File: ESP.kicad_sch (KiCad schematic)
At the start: 13 parts, among them J1 Conn_01x03, SW1 SW_Push, U1 RP2040, U5 W25X40CLSS, U6 DRV8833PW, U7 DRV8833PW, U8 DRV8833PW

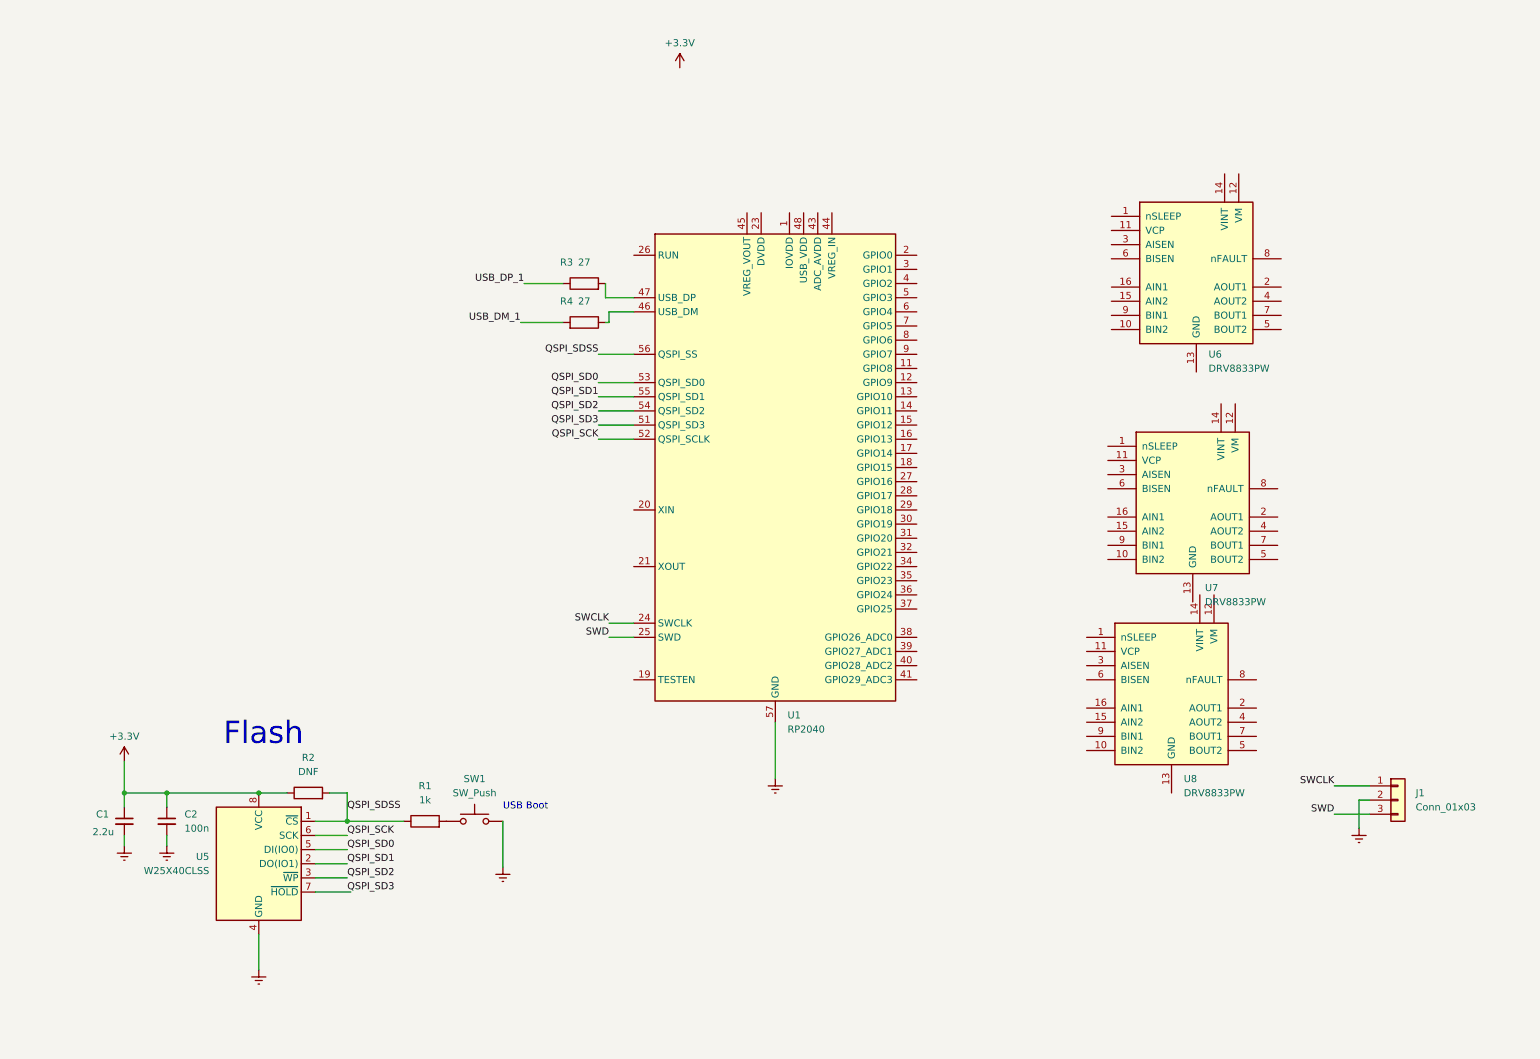
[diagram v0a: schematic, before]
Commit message: More progress
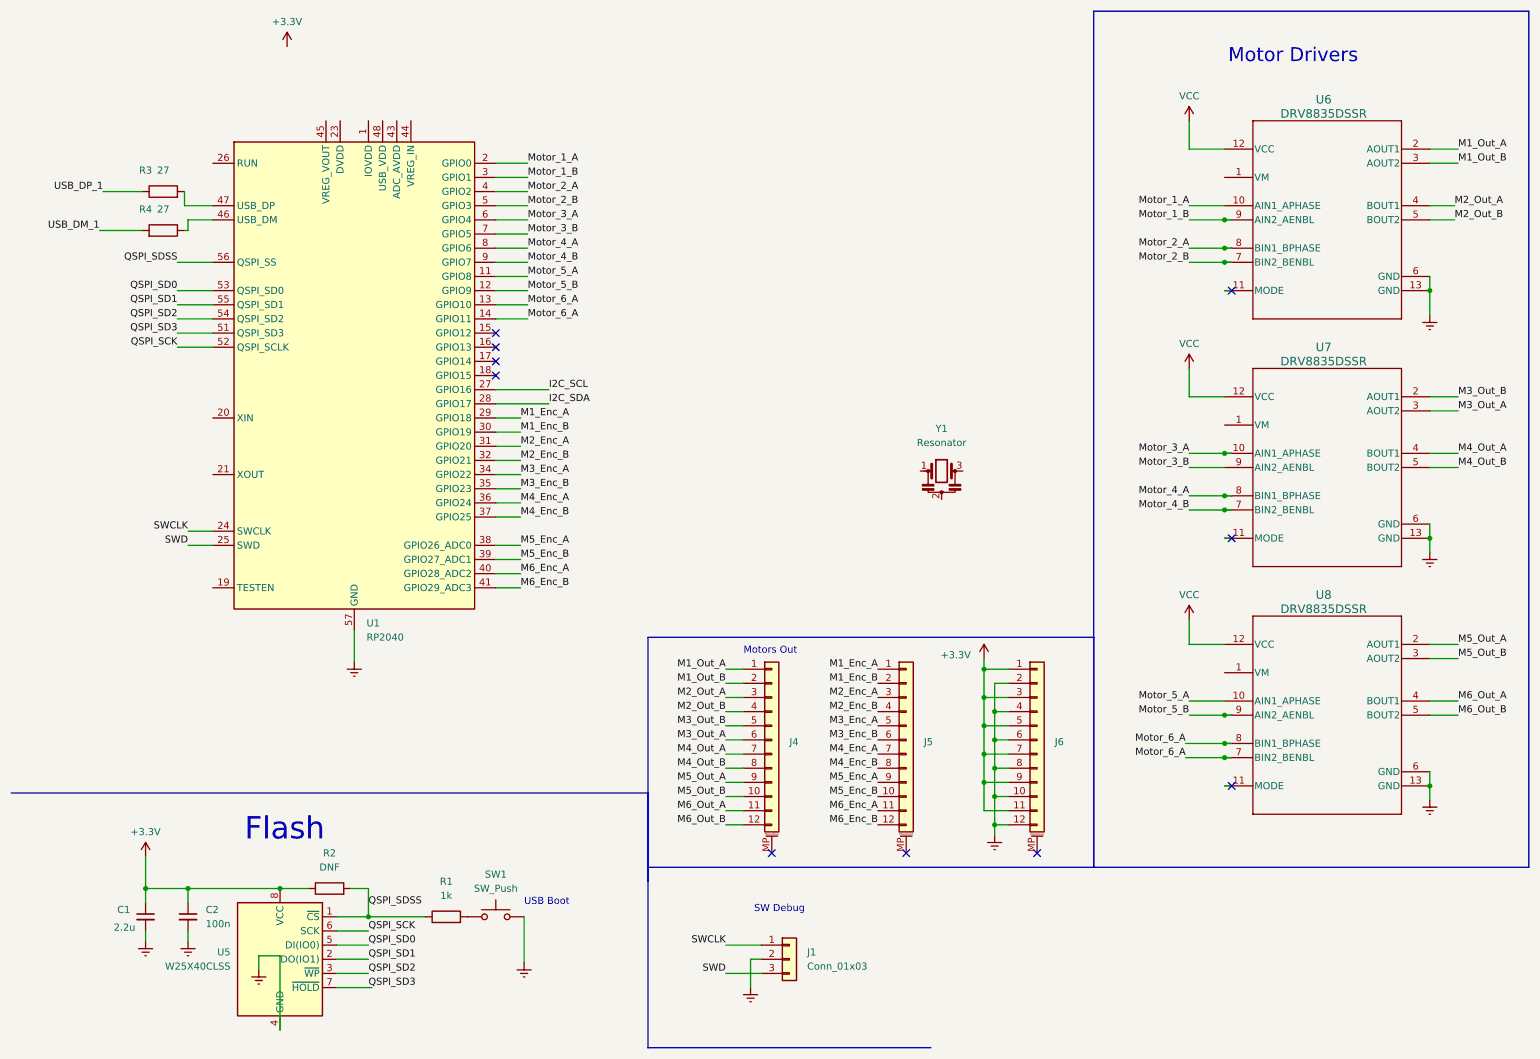
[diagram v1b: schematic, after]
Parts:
- removed U6, U7, U8: DRV8833PW, Package_SO:TSSOP-16_4.4x5mm_P0.65mm, symbol Driver_Motor:DRV8833PW
- added J4, J5, J6: Conn_01x12_MountingPin, symbol Connector_Generic_MountingPin:Conn_01x12_MountingPin
- added U6, U7, U8: DRV8835DSSR, DSS0012A, symbol DRV8835:DRV8835DSSR
- added Y1: Resonator, symbol Device:Resonator
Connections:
- net +3.3V: now also J6.1 (Pin_1), J6.11 (Pin_11), J6.3 (Pin_3), J6.5 (Pin_5), J6.7 (Pin_7), J6.9 (Pin_9)
- net Earth: now also J6.10 (Pin_10), J6.12 (Pin_12), J6.2 (Pin_2), J6.4 (Pin_4), J6.6 (Pin_6), J6.8 (Pin_8), U6.13 (GND), U6.6 (GND), U7.13 (GND), U7.6 (GND), U8.13 (GND), U8.6 (GND)
- net Motor_5_A: now reaches U1.11 (GPIO8)
- net Motor_5_A: now also U8.10 (AIN1_APHASE)
- net Motor_5_B: now reaches U1.12 (GPIO9)
- net Motor_5_B: now also U8.9 (AIN2_AENBL)
- net Motor_6_A: now reaches U1.13 (GPIO10)
- net Motor_6_A: now also U1.14 (GPIO11), U8.7 (BIN2_BENBL), U8.8 (BIN1_BPHASE)
- net Motor_1_A: now reaches U1.2 (GPIO0)
- net Motor_1_A: now also U6.10 (AIN1_APHASE)
- net I2C_SCL: now reaches U1.27 (GPIO16)
- net I2C_SDA: now reaches U1.28 (GPIO17)
- net M1_Enc_A: now reaches U1.29 (GPIO18)
- net M1_Enc_A: now also J5.1 (Pin_1)
- net Motor_1_B: now reaches U1.3 (GPIO1)
- net Motor_1_B: now also U6.9 (AIN2_AENBL)
- net M1_Enc_B: now reaches U1.30 (GPIO19)
- net M1_Enc_B: now also J5.2 (Pin_2)
- net M2_Enc_A: now reaches U1.31 (GPIO20)
- net M2_Enc_A: now also J5.3 (Pin_3)
- net M2_Enc_B: now reaches U1.32 (GPIO21)
- net M2_Enc_B: now also J5.4 (Pin_4)
- net M3_Enc_A: now reaches U1.34 (GPIO22)
- net M3_Enc_A: now also J5.5 (Pin_5)
- net M3_Enc_B: now reaches U1.35 (GPIO23)
- net M3_Enc_B: now also J5.6 (Pin_6)
- net M4_Enc_A: now reaches U1.36 (GPIO24)
- net M4_Enc_A: now also J5.7 (Pin_7)
- net M4_Enc_B: now reaches U1.37 (GPIO25)
- net M4_Enc_B: now also J5.8 (Pin_8)
- net M5_Enc_A: now reaches U1.38 (GPIO26_ADC0)
- net M5_Enc_A: now also J5.9 (Pin_9)
- net M5_Enc_B: now reaches U1.39 (GPIO27_ADC1)
- net M5_Enc_B: now also J5.10 (Pin_10)
- net Motor_2_A: now reaches U1.4 (GPIO2)
- net Motor_2_A: now also U6.8 (BIN1_BPHASE)
- net M6_Enc_A: now reaches U1.40 (GPIO28_ADC2)
- net M6_Enc_A: now also J5.11 (Pin_11)
- net M6_Enc_B: now reaches U1.41 (GPIO29_ADC3)
- net M6_Enc_B: now also J5.12 (Pin_12)
- net Motor_2_B: now reaches U1.5 (GPIO3)
- net Motor_2_B: now also U6.7 (BIN2_BENBL)
- net Motor_3_A: now reaches U1.6 (GPIO4)
- net Motor_3_A: now also U7.10 (AIN1_APHASE)
- net Motor_3_B: now reaches U1.7 (GPIO5)
- net Motor_3_B: now also U7.9 (AIN2_AENBL)
- net Motor_4_A: now reaches U1.8 (GPIO6)
- net Motor_4_A: now also U7.8 (BIN1_BPHASE)
- net Motor_4_B: now reaches U1.9 (GPIO7)
- net Motor_4_B: now also U7.7 (BIN2_BENBL)
- new net M1_Out_A: J4.1 (Pin_1), U6.2 (AOUT1)
- new net M1_Out_B: J4.2 (Pin_2), U6.3 (AOUT2)
- new net M2_Out_A: J4.3 (Pin_3), U6.4 (BOUT1)
- new net M2_Out_B: J4.4 (Pin_4), U6.5 (BOUT2)
- new net M3_Out_A: J4.6 (Pin_6), U7.3 (AOUT2)
- new net M3_Out_B: J4.5 (Pin_5), U7.2 (AOUT1)
- new net M4_Out_A: J4.7 (Pin_7), U7.4 (BOUT1)
- new net M4_Out_B: J4.8 (Pin_8), U7.5 (BOUT2)
- new net M5_Out_A: J4.9 (Pin_9), U8.2 (AOUT1)
- new net M5_Out_B: J4.10 (Pin_10), U8.3 (AOUT2)
- new net M6_Out_A: J4.11 (Pin_11), U8.4 (BOUT1)
- new net M6_Out_B: J4.12 (Pin_12), U8.5 (BOUT2)
- new net VCC: U6.12 (VCC), U7.12 (VCC), U8.12 (VCC)
- no-connect marks 0 -> 10
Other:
- note added: "Motor Drivers"
- note added: "Motors Out"
- note added: "SW Debug"
- moved on the sheet: C1, C2, J1, R1, R2, R3, R4, SW1, U1, U5

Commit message: More Progress
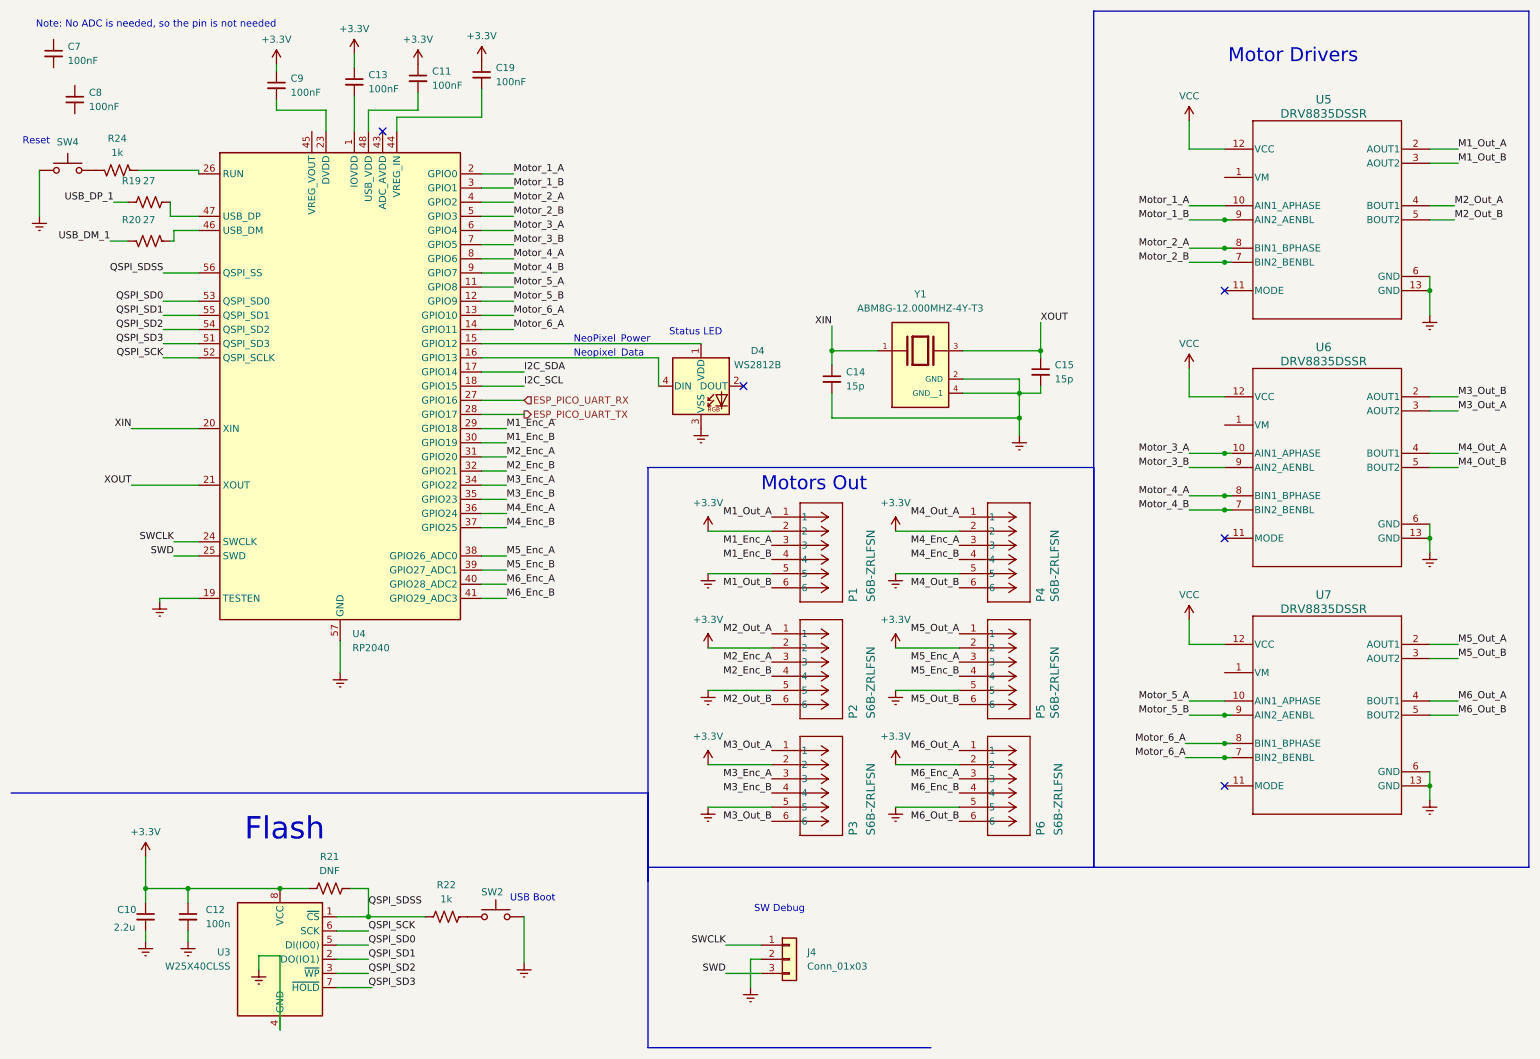
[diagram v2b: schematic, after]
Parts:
- removed J4, J5, J6: Conn_01x12_MountingPin, symbol Connector_Generic_MountingPin:Conn_01x12_MountingPin
- removed Y1: Resonator, symbol Device:Resonator
- added C11, C13, C19, C7, C8, C9: 100nF, symbol Device:C_Small
- added C14, C15: 15p, symbol Device:C_Small
- added D4: WS2812B, LED_SMD:LED_WS2812B_PLCC4_5.0x5.0mm_P3.2mm, symbol LED:WS2812B
- added P1, P2, P3, P4, P5, P6: S6B-ZRLFSN, S6B-ZR_JST, symbol JST-ZH:S6B-ZRLFSN
- added R24: 1k, Resistor_SMD:R_0612_1632Metric, symbol Device:R_US
- added SW4: SW_Push, symbol Switch:SW_Push
- added Y1: ABM8G-12.000MHZ-4Y-T3, ABM8G-12.000MHZ-4Y-T3:XTAL_ABM8G-12.000MHZ-4Y-T3, symbol ABMG8_12:ABM8G-12.000MHZ-4Y-T3
- R19: renamed from R3; symbol Device:R -> Device:R_US
- R20: renamed from R4; symbol Device:R -> Device:R_US
- R21: renamed from R2; symbol Device:R -> Device:R_US
- R22: renamed from R1; symbol Device:R -> Device:R_US
- renumbered C1 to C10, C2 to C12, J1 to J4, SW1 to SW2, U5 to U3, U1 to U4, U6 to U5, U7 to U6, U8 to U7
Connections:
- net +3.3V: now also C11.1, C13.1, C19.1, C9.1, P1.2, P2.2, P3.2, P4.2, P5.2, P6.2
- net Earth: now also U4.19 (TESTEN), C14.2, C15.2, D4.3 (VSS), P1.5, P2.5, P3.5, P4.5, P5.5, P6.5, SW4.2, Y1.2 (GND), Y1.4 (GND__1)
- net I2C_SCL: now also U4.18 (GPIO15); no longer U4.27 (GPIO16)
- net I2C_SDA: now also U4.17 (GPIO14); no longer U4.28 (GPIO17)
- net M1_Enc_A: now also P1.3
- net M1_Enc_B: now also P1.4
- net M1_Out_A: now also P1.1
- net M1_Out_B: now also P1.6
- net M2_Enc_A: now also P2.3
- net M2_Enc_B: now also P2.4
- net M2_Out_A: now also P2.1
- net M2_Out_B: now also P2.6
- net M3_Enc_A: now also P3.3
- net M3_Enc_B: now also P3.4
- net M3_Out_A: now also P3.1
- net M3_Out_B: now also P3.6
- net M4_Enc_A: now also P4.3
- net M4_Enc_B: now also P4.4
- net M4_Out_A: now also P4.1
- net M4_Out_B: now also P4.6
- net M5_Enc_A: now also P5.3
- net M5_Enc_B: now also P5.4
- net M5_Out_A: now also P5.1
- net M5_Out_B: now also P5.6
- net M6_Enc_A: now also P6.3
- net M6_Enc_B: now also P6.4
- net M6_Out_A: now also P6.1
- net M6_Out_B: now also P6.6
- net at U4.1 (IOVDD), U4.10 (IOVDD), U4.22 (IOVDD)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: now also C13.2
- net at U4.15 (GPIO12): now also D4.1 (VDD)
- net at U4.16 (GPIO13): now also D4.4 (DIN)
- net XIN: now reaches U4.20 (XIN)
- net XIN: now also C14.1, Y1.1
- net XOUT: now reaches U4.21 (XOUT)
- net XOUT: now also C15.1, Y1.3
- net at U4.23 (DVDD), U4.50 (DVDD): now also C9.2
- net at U4.26 (RUN): now also R24.1
- net at U4.44 (VREG_IN): now also C19.2
- net at U4.48 (USB_VDD): now also C11.2
- new net: R24.2, SW4.1
- new net ESP_PICO_UART_RX: U4.27 (GPIO16)
- new net ESP_PICO_UART_TX: U4.28 (GPIO17)
- no-connect marks 10 -> 5
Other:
- note added: "NeoPixel_Power"
- note added: "Neopixel_Data"
- note added: "Note: No ADC is needed, so the pin is not needed"
- note added: "Reset"
- note added: "Status LED"
- moved on the sheet: U4
